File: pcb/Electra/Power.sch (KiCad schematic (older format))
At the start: 26 parts, among them J201 8-28V, J202 USB, J203 Enable VIn, U201 AMS1117-3.3, U202 TPS54202DDCR

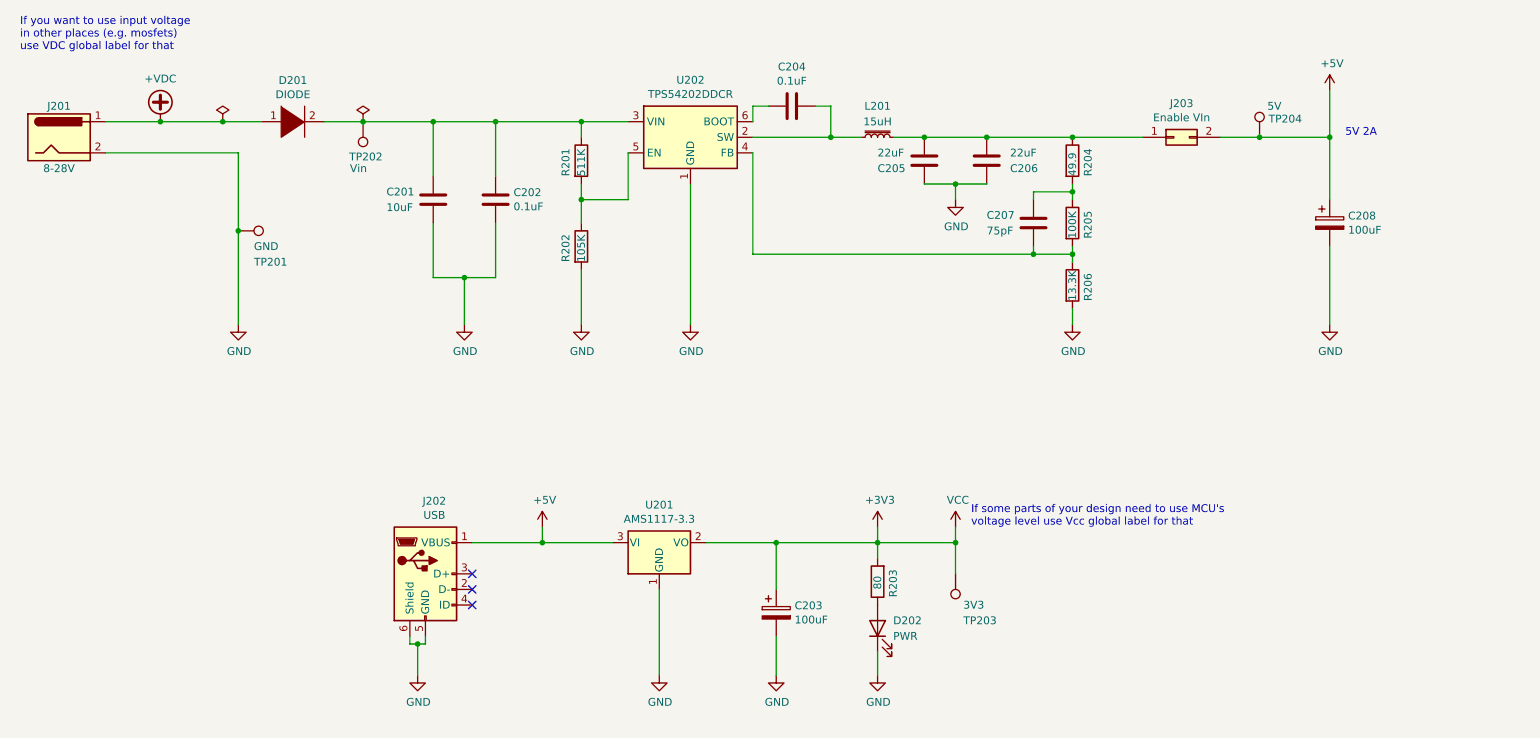
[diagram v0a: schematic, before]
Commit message: Rev 2 completed, todo check all and remove not needed filed
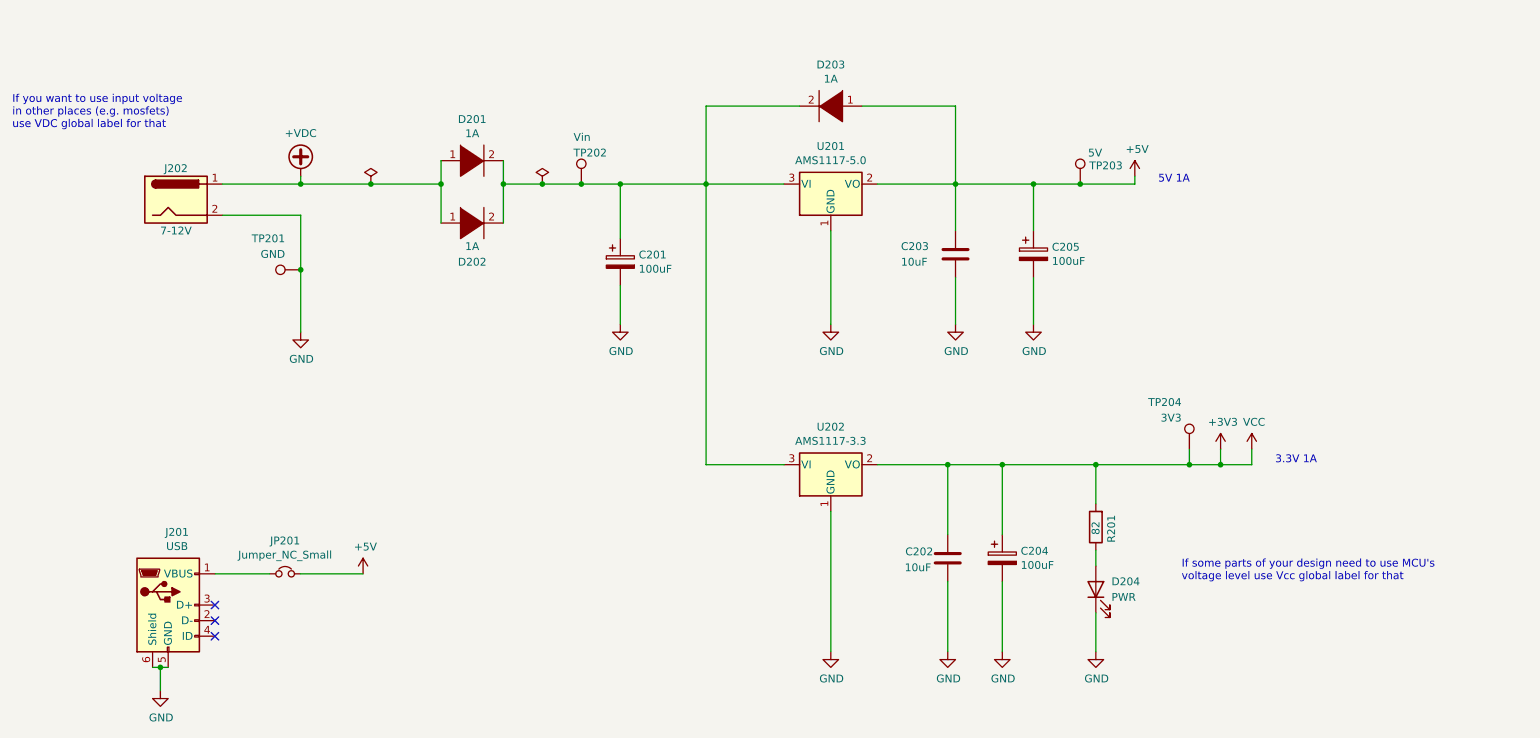
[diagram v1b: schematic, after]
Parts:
- removed C201: 10uF, Capacitor_SMD:C_1210_3225Metric_Pad1.33x2.70mm_HandSolder, symbol Device:C
- removed C203, C208: 100uF, Capacitor_SMD:CP_Elec_5x5.4, symbol Device:CP
- removed C204: 0.1uF, Capacitor_SMD:C_0603_1608Metric_Pad1.08x0.95mm_HandSolder, symbol Device:C
- removed C205, C206: 22uF, Capacitor_SMD:C_1210_3225Metric_Pad1.33x2.70mm_HandSolder, symbol Device:C
- removed C207: 75pF, Capacitor_SMD:C_0603_1608Metric_Pad1.08x0.95mm_HandSolder, symbol Device:C
- removed D202: PWR, LED_SMD:LED_0603_1608Metric_Pad1.05x0.95mm_HandSolder, symbol Device:LED
- removed J201: 8-28V, Connector_BarrelJack:BarrelJack_Horizontal, symbol Connector:Barrel_Jack
- removed J202: USB, Connector_USB:USB_Micro-B_Molex-105017-0001, symbol Connector:USB_B_Micro
- removed J203: Enable VIn, Connector_PinHeader_2.54mm:PinHeader_2x01_P2.54mm_Vertical, symbol Connector_Generic:Conn_02x01
- removed L201: 15uH, Inductor_SMD:L_10.4x10.4_H4.8, symbol Device:L_Core_Iron_Small
- removed R202: 105K, Resistor_SMD:R_0603_1608Metric_Pad0.98x0.95mm_HandSolder, symbol Device:R
- removed R203: 80, Resistor_SMD:R_0603_1608Metric_Pad0.98x0.95mm_HandSolder, symbol Device:R
- removed R204: 49.9, Resistor_SMD:R_0603_1608Metric_Pad0.98x0.95mm_HandSolder, symbol Device:R
- removed R205: 100K, Resistor_SMD:R_0603_1608Metric_Pad0.98x0.95mm_HandSolder, symbol Device:R
- removed R206: 13.3K, Resistor_SMD:R_0603_1608Metric_Pad0.98x0.95mm_HandSolder, symbol Device:R
- removed U201: AMS1117-3.3, Package_TO_SOT_SMD:SOT-223-3_TabPin2, symbol Regulator_Linear:AMS1117-3.3
- removed U202: TPS54202DDCR, Package_TO_SOT_SMD:SOT-23-6, symbol Regulator_Switching:TPS54202DDC
- added C201, C204, C205: 100uF, Capacitor_SMD:CP_Elec_6.3x5.4, symbol Device:CP
- added C203: 10uF, Capacitor_SMD:C_0805_2012Metric_Pad1.18x1.45mm_HandSolder, symbol Device:C
- added D202, D203: 1A, Diode_SMD:D_SMA_Handsoldering, symbol pspice:DIODE
- added D204: PWR, LED_SMD:LED_0603_1608Metric_Pad1.05x0.95mm_HandSolder, symbol Device:LED
- added J201: USB, Connector_USB:USB_Micro-B_Molex-105017-0001, symbol Connector:USB_B_Micro
- added J202: 7-12V, Connector_BarrelJack:BarrelJack_Horizontal, symbol Connector:Barrel_Jack
- added JP201: Jumper_NC_Small, Jumper:SolderJumper-2_P1.3mm_Bridged_RoundedPad1.0x1.5mm, symbol Device:Jumper_NC_Small
- added U201: AMS1117-5.0, Package_TO_SOT_SMD:SOT-223-3_TabPin2, symbol Regulator_Linear:AMS1117-5.0
- added U202: AMS1117-3.3, Package_TO_SOT_SMD:SOT-223-3_TabPin2, symbol Regulator_Linear:AMS1117-3.3
- C202: value 0.1uF -> 10uF; footprint Capacitor_SMD:C_0603_1608Metric_Pad1.08x0.95mm_HandSolder -> Capacitor_SMD:C_0805_2012Metric_Pad1.18x1.45mm_HandSolder; Description 100nF ±10% 25V X7R 0603 Multilayer Ceramic Capacitors MLCC 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 -> (none); LCSC (none) -> C15850; LCSC Part # C92490 -> (none); Manufacturer YAGEO -> (none); Maximum Value 25V -> (none); Maximum value (none) -> 25V; Mfr.Part # CC0603KRX7R8BB104 -> (none); Package Reference 0603 -> (none)
- D201: value DIODE -> 1A; footprint Diode_SMD:D_SMA -> Diode_SMD:D_SMA_Handsoldering; Description 1kV 2A 1.1V @ 2A SMA(DO-214AC) Diodes - General Purpose RoHS -> (none); LCSC (none) -> C95872; LCSC Part # C18905 -> (none); Manufacturer MDD(Microdiode Electronics) -> (none); Maximum Value 2A -> 1A; Mfr.Part # S2M -> (none)
- R201: value 511K -> 82; Description 511kΩ ±1% 0.1W ±100ppm/℃ 0603 Chip Resistor - Surface Mount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 -> (none); LCSC (none) -> C23255; LCSC Part # C23194 -> (none); Manufacturer UNI-ROYAL(Uniroyal Elec) -> (none); Mfr.Part # 0603WAF5113T5E -> (none)
- TP201, TP202: Description - -> (none); LCSC Part # - -> (none); Manufacturer - -> (none); Mfr.Part # - -> (none)
- TP203: value 3V3 -> 5V; Description - -> (none); LCSC Part # - -> (none); Manufacturer - -> (none); Mfr.Part # - -> (none)
- TP204: value 5V -> 3V3; Description - -> (none); LCSC Part # - -> (none); Manufacturer - -> (none); Mfr.Part # - -> (none)
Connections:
- net +3V3: now also C202.1, R201.2, TP204.1, C204.1, U202.2 (VO); no longer TP203.1
- net +5V: now also TP203.1, C203.1, C205.1, D203.1 (K), JP201.2, U201.2 (VO); no longer TP204.1
- net +VDC: now also D202.1 (K), J202.1
- net GND: now also C201.2, C203.2, C204.2, C205.2, D204.1 (K), J201.5 (GND), J201.6 (Shield), J202.2, U201.1 (GND), U202.1 (GND)
- net at D201.2 (A), TP202.1: now also C201.1, D202.2 (A), D203.2 (A), U201.3 (VI), U202.3 (VI); no longer C202.1, R201.1
- new net: J201.1 (VBUS), JP201.1
- new net: D204.2 (A), R201.1
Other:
- note added: "3.3V 1A"
- note added: "5V 1A"
- note removed: "5V 2A"
